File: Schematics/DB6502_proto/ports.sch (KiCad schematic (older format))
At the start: 20 parts, among them J1 Power plug, J10 System Bus, J2 Controls, J3 AVR ISP, J4 Debug USB, J5 JPR, J6 Debug UART, J7 UART A, J8 UART B, J9 I/O Bus

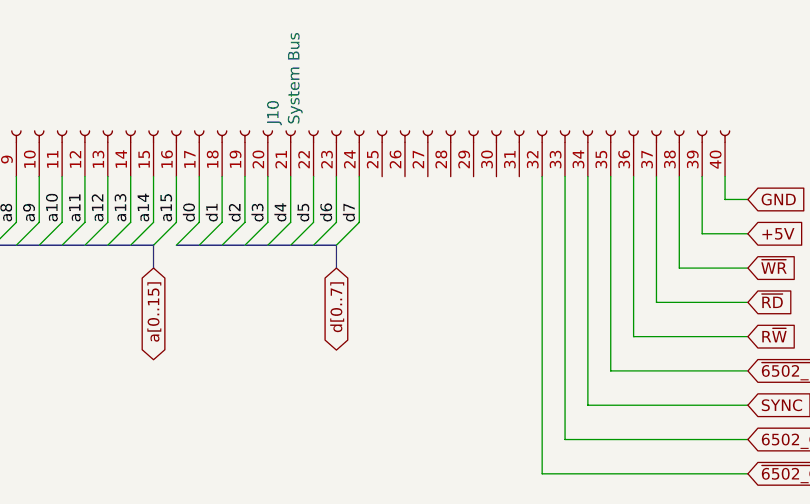
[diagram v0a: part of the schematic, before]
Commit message: Further improvements
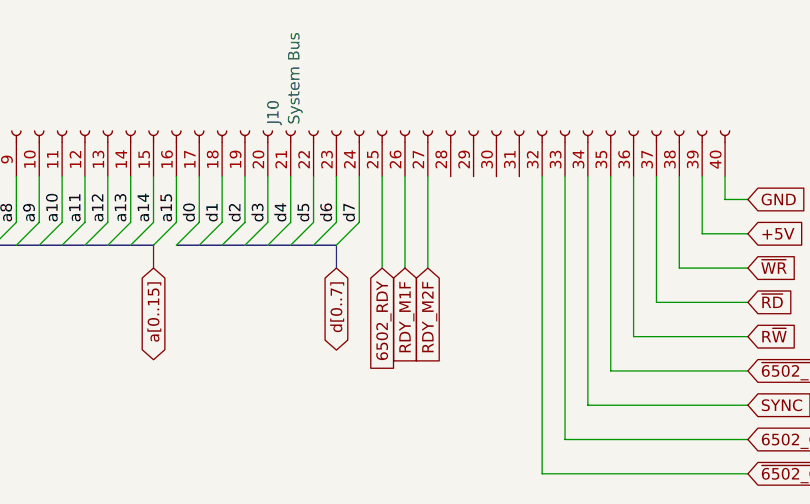
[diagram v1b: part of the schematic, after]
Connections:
- net 6502_RDY: now also J10.25 (Pin_25)
- net RDY_M1F: now also J10.26 (Pin_26)
- net RDY_M2F: now also J10.27 (Pin_27)
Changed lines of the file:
@@
 Text GLabel 2950 5000 3    50   Input ~ 0
 GND
+Text GLabel 4900 6800 3    50   Input ~ 0
+RDY_M1F
+Text GLabel 5000 6800 3    50   Input ~ 0
+RDY_M2F
+Wire Wire Line
+	4800 6800 4800 6400
+Wire Wire Line
+	4900 6800 4900 6400
+Text GLabel 4800 6800 3    50   Input ~ 0
+6502_RDY
+Wire Wire Line
+	5000 6800 5000 6400
 Wire Bus Line
 	10750 2150 10750 2350
